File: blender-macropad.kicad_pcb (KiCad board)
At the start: 2 copper layers, 80 x 90 mm, 29 parts, among them J1 Conn_02x12_Counter_Clockwise, J2 Conn_01x07, SW1 SW_Push, SW10 SW_Push, SW11 SW_Push, SW12 SW_Push, SW13 RotaryEncoder_Switch, SW2 SW_Push, SW3 SW_Push, SW4 SW_Push, SW5 SW_Push, SW6 SW_Push, SW7 SW_Push, SW8 SW_Push, SW9 SW_Push

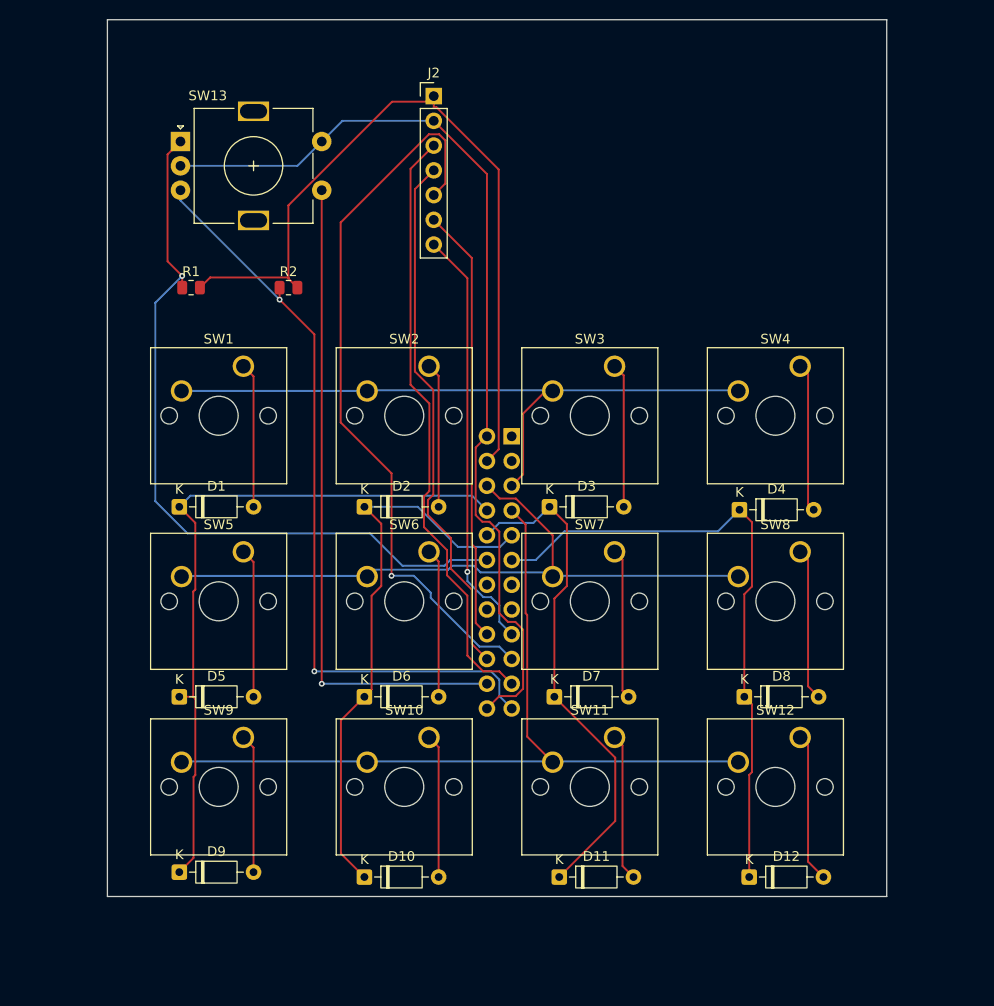
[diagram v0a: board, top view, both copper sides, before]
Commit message: Updated PCB
Fixed PCB
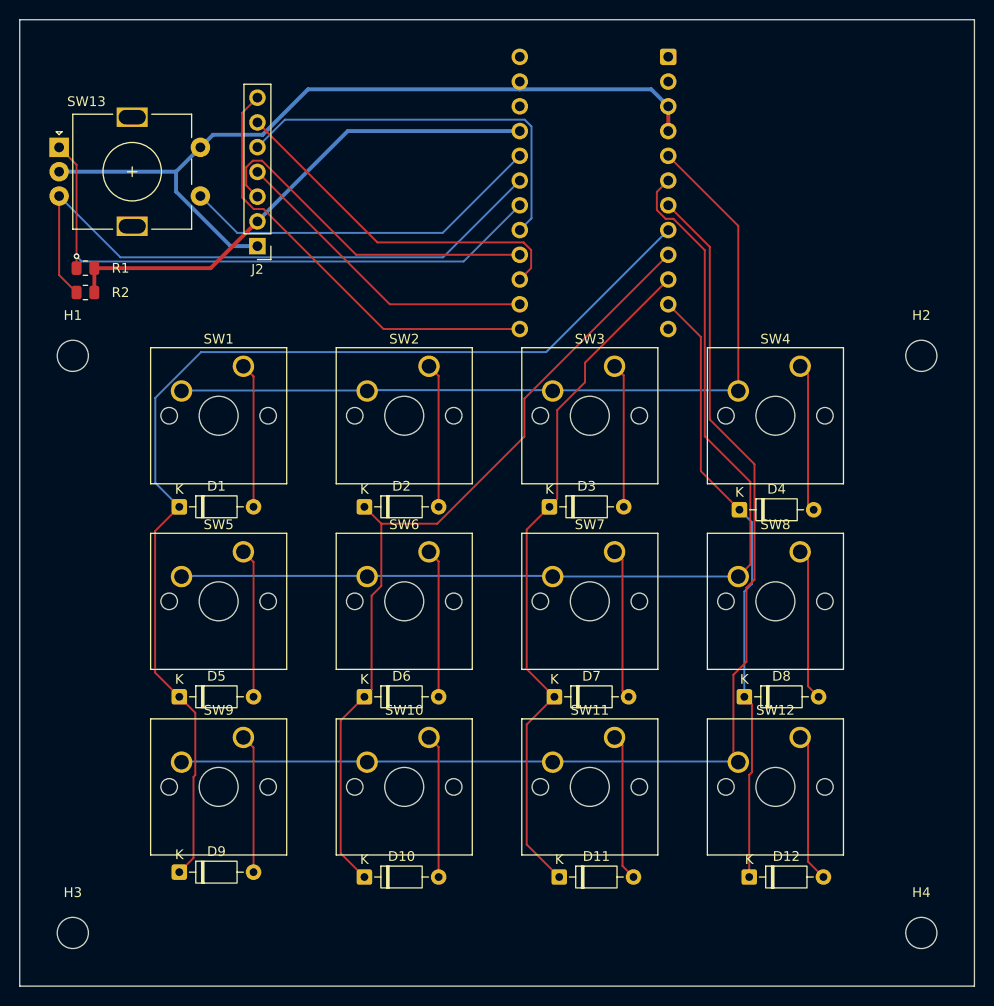
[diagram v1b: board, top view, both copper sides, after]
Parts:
- added H1: M3, MountingHole_3.2mm_M3, F.Cu at (170.4, 51.0)
- added H2: M3, MountingHole_3.2mm_M3, F.Cu at (257.6, 51.0)
- added H3: M3, MountingHole_3.2mm_M3, F.Cu at (170.4, 110.2)
- added H4: M3, MountingHole_3.2mm_M3, F.Cu at (257.6, 110.2)
- J1: footprint Connector_PinHeader_2.54mm:PinHeader_2x12_P2.54mm_Vertical -> Package_DIP:DIP-24_W15.24mm
- moved J1 42.1 mm to (231.6, 20.3)
- moved J2 23.8 mm to (189.4, 39.7), turned to 180 degrees
- moved R2 20.8 mm to (171.7, 44.5)
- moved SW13 12.5 mm to (169.0, 29.6)
- moved R1 11.0 mm to (171.7, 42.0)
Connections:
- J1 pad 1: /RAW -> unconnected-(J1-Pin_1-Pad1)
- J1 pad 12: /ENC_A -> unconnected-(J1-Pin_12-Pad12)
- J1 pad 13: unconnected-(J1-Pin_13-Pad13) -> /OLED_CS
- J1 pad 14: unconnected-(J1-Pin_14-Pad14) -> /OLED_MOSI
- J1 pad 15: unconnected-(J1-Pin_15-Pad15) -> /OLED_DC
- J1 pad 16: unconnected-(J1-Pin_16-Pad16) -> /OLED_CLK
- J1 pad 18: /OLED_DC -> /ENC_A
- J1 pad 19: /OLED_CS -> /ENC_B
- J1 pad 2: /GND -> unconnected-(J1-Pin_2-Pad2)
- J1 pad 20: /OLED_CLK -> /ENC_SW
- J1 pad 21: /OLED_MOSI -> /VCC
- J1 pad 22: /ENC_SW -> unconnected-(J1-Pin_22-Pad22)
- J1 pad 23: /ENC_B -> /GND
- J1 pad 24: /GND -> unconnected-(J1-Pin_24-Pad24)
- J1 pad 3: /RST -> /GND
- J1 pad 4: /VCC -> /GND
- J2 pad 1: /VCC -> /GND
- J2 pad 2: /GND -> /VCC
- J2 pad 3: /OLED_MOSI -> /OLED_CLK
- J2 pad 4: /OLED_CLK -> /OLED_MOSI
- J2 pad 5: /OLED_CS -> /OLED_RST
- J2 pad 7: /OLED_RST -> /OLED_CS
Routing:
- net /COL0: track 73.2 -> 112.9 mm
- net /ROW2: track 84.9 -> 119.3 mm
- net /ROW1: track 71.3 -> 103.4 mm
- net /OLED_CS: track 75.5 -> 45.0 mm, vias 1 -> 0
- net /ENC_SW: track 67.6 -> 37.6 mm, vias 1 -> 0
- net /OLED_MOSI: track 62.0 -> 32.6 mm
- net /VCC: track 78.6 -> 52.0 mm
- net /COL1: track 58.8 -> 84.6 mm
- net /COL2: track 51.9 -> 71.1 mm
- net /OLED_CLK: track 54.5 -> 35.9 mm
- net /ENC_A: track 77.5 -> 61.2 mm
- net /ENC_B: track 79.1 -> 63.8 mm, vias 2 -> 0
- net /ROW0: track 69.2 -> 84.4 mm
- net /GND: track 96.4 -> 82.8 mm
- net /OLED_DC: track 44.8 -> 37.0 mm
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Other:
- board size 80 x 90 mm -> 98 x 99.2 mm
- board text added: "OLED 2.08" 72.5x27.24"
- board text added: "PARTS FACE OUT"
- board text added: "Pro Micro RP2040 (B) 17.78x33.02"
- board text added: "RAW"
- board text added: "TX0"
